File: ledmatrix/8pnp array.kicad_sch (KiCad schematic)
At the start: 8 parts

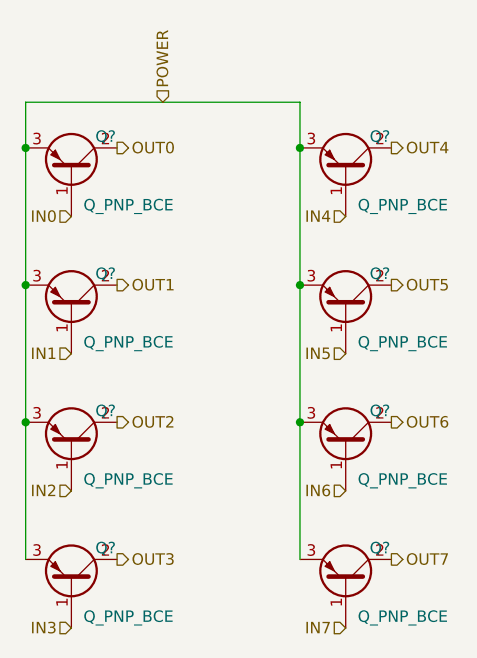
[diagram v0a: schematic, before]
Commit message: Finish ledmatrix pcb reverse engineering.
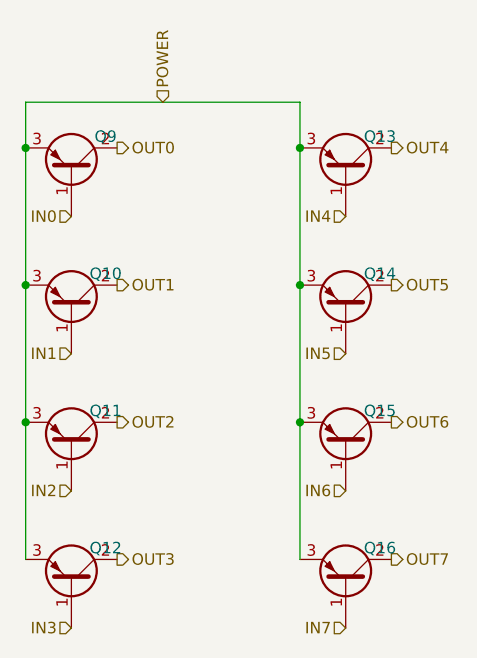
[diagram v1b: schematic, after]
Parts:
- removed Q? (x8): Q_PNP_BCE, symbol Device:Q_PNP_BCE
- added Q10, Q11, Q12, Q13, Q14, Q15, Q16, Q9: (no value), symbol Device:Q_PNP_BCE
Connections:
- net IN0: now also Q9.1 (B)
- net IN1: now also Q10.1 (B)
- net IN2: now also Q11.1 (B)
- net IN3: now also Q12.1 (B)
- net IN4: now also Q13.1 (B)
- net IN5: now also Q14.1 (B)
- net IN6: now also Q15.1 (B)
- net IN7: now also Q16.1 (B)
- net OUT0: now also Q9.2 (C)
- net OUT1: now also Q10.2 (C)
- net OUT2: now also Q11.2 (C)
- net OUT3: now also Q12.2 (C)
- net OUT4: now also Q13.2 (C)
- net OUT5: now also Q14.2 (C)
- net OUT6: now also Q15.2 (C)
- net OUT7: now also Q16.2 (C)
- net POWER: now also Q10.3 (E), Q11.3 (E), Q12.3 (E), Q13.3 (E), Q14.3 (E), Q15.3 (E), Q16.3 (E), Q9.3 (E)
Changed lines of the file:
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@@
     (effects (font (size 1.27 1.27)) (justify right))
+  )
+  (symbol (lib_id "Device:Q_PNP_BCE") (at 123.19 44.45 270) (mirror x) (unit 1)
+    (in_bom yes) (on_board yes)
+    (property "Reference" "Q13" (id 0) (at 127 40.64 90))
+    (property "Value" "" (id 1) (at 129.54 48.26 90))
+    (property "Footprint" "" (id 2) (at 125.73 39.37 0)
+      (effects (font (size 1.27 1.27)) hide)
+    )
+    (property "Datasheet" "~" (id 3) (at 123.19 44.45 0)
+      (effects (font (size 1.27 1.27)) hide)
+    )
+    (pin "1")
+    (pin "2")
+    (pin "3")
+  )
+  (symbol (lib_id "Device:Q_PNP_BCE") (at 123.19 59.69 270) (mirror x) (unit 1)
+    (in_bom yes) (on_board yes)
+    (property "Reference" "Q14" (id 0) (at 127 55.88 90))
+    (property "Value" "" (id 1) (at 129.54 63.5 90))
+    (property "Footprint" "" (id 2) (at 125.73 54.61 0)
+      (effects (font (size 1.27 1.27)) hide)
+    )
+    (property "Datasheet" "~" (id 3) (at 123.19 59.69 0)
+      (effects (font (size 1.27 1.27)) hide)
+    )
+    (pin "1")
+    (pin "2")
+    (pin "3")
+  )
+  (symbol (lib_id "Device:Q_PNP_BCE") (at 123.19 90.17 270) (mirror x) (unit 1)
+    (in_bom yes) (on_board yes)
+    (property "Reference" "Q16" (id 0) (at 127 86.36 90))
+    (property "Value" "" (id 1) (at 129.54 93.98 90))
+    (property "Footprint" "" (id 2) (at 125.73 85.09 0)
+      (effects (font (size 1.27 1.27)) hide)
+    )
+    (property "Datasheet" "~" (id 3) (at 123.19 90.17 0)
+      (effects (font (size 1.27 1.27)) hide)
+    )
+    (pin "1")
+    (pin "2")
+    (pin "3")
   )
   (symbol (lib_id "Device:Q_PNP_BCE") (at 92.71 44.45 270) (mirror x) (unit 1)
     (in_bom yes) (on_board yes)
-    (property "Reference" "Q?" (id 0) (at 96.52 40.64 90))
-    (property "Value" "Q_PNP_BCE" (id 1) (at 99.06 48.26 90))
+    (property "Reference" "Q9" (id 0) (at 96.52 40.64 90))
+    (property "Value" "" (id 1) (at 99.06 48.26 90))
     (property "Footprint" "" (id 2) (at 95.25 39.37 0)
       (effects (font (size 1.27 1.27)) hide)
@@
     (pin "3")
   )
-  (symbol (lib_id "Device:Q_PNP_BCE") (at 123.19 59.69 270) (mirror x) (unit 1)
+  (symbol (lib_id "Device:Q_PNP_BCE") (at 92.71 90.17 270) (mirror x) (unit 1)
     (in_bom yes) (on_board yes)
-    (property "Reference" "Q?" (id 0) (at 127 55.88 90))
-    (property "Value" "Q_PNP_BCE" (id 1) (at 129.54 63.5 90))
-    (property "Footprint" "" (id 2) (at 125.73 54.61 0)
+    (property "Reference" "Q12" (id 0) (at 96.52 86.36 90))
+    (property "Value" "" (id 1) (at 99.06 93.98 90))
+    (property "Footprint" "" (id 2) (at 95.25 85.09 0)
       (effects (font (size 1.27 1.27)) hide)
     )
-    (property "Datasheet" "~" (id 3) (at 123.19 59.69 0)
-      (effects (font (size 1.27 1.27)) hide)
-    )
-    (pin "1")
-    (pin "2")
-    (pin "3")
-  )
-  (symbol (lib_id "Device:Q_PNP_BCE") (at 92.71 74.93 270) (mirror x) (unit 1)
-    (in_bom yes) (on_board yes)
-    (property "Reference" "Q?" (id 0) (at 96.52 71.12 90))
-    (property "Value" "Q_PNP_BCE" (id 1) (at 99.06 78.74 90))
-    (property "Footprint" "" (id 2) (at 95.25 69.85 0)
-      (effects (font (size 1.27 1.27)) hide)
-    )
-    (property "Datasheet" "~" (id 3) (at 92.71 74.93 0)
+    (property "Datasheet" "~" (id 3) (at 92.71 90.17 0)
       (effects (font (size 1.27 1.27)) hide)
     )
@@
   (symbol (lib_id "Device:Q_PNP_BCE") (at 92.71 59.69 270) (mirror x) (unit 1)
     (in_bom yes) (on_board yes)
-    (property "Reference" "Q?" (id 0) (at 96.52 55.88 90))
-    (property "Value" "Q_PNP_BCE" (id 1) (at 99.06 63.5 90))
+    (property "Reference" "Q10" (id 0) (at 96.52 55.88 90))
+    (property "Value" "" (id 1) (at 99.06 63.5 90))
     (property "Footprint" "" (id 2) (at 95.25 54.61 0)
       (effects (font (size 1.27 1.27)) hide)
@@
     (pin "3")
   )
-  (symbol (lib_id "Device:Q_PNP_BCE") (at 92.71 90.17 270) (mirror x) (unit 1)
-    (in_bom yes) (on_board yes)
-    (property "Reference" "Q?" (id 0) (at 96.52 86.36 90))
-    (property "Value" "Q_PNP_BCE" (id 1) (at 99.06 93.98 90))
-    (property "Footprint" "" (id 2) (at 95.25 85.09 0)
-      (effects (font (size 1.27 1.27)) hide)
-    )
-    (property "Datasheet" "~" (id 3) (at 92.71 90.17 0)
-      (effects (font (size 1.27 1.27)) hide)
-    )
-    (pin "1")
-    (pin "2")
-    (pin "3")
-  )
-  (symbol (lib_id "Device:Q_PNP_BCE") (at 123.19 90.17 270) (mirror x) (unit 1)
-    (in_bom yes) (on_board yes)
-    (property "Reference" "Q?" (id 0) (at 127 86.36 90))
-    (property "Value" "Q_PNP_BCE" (id 1) (at 129.54 93.98 90))
-    (property "Footprint" "" (id 2) (at 125.73 85.09 0)
-      (effects (font (size 1.27 1.27)) hide)
-    )
-    (property "Datasheet" "~" (id 3) (at 123.19 90.17 0)
-      (effects (font (size 1.27 1.27)) hide)
-    )
-    (pin "1")
-    (pin "2")
-    (pin "3")
-  )
   (symbol (lib_id "Device:Q_PNP_BCE") (at 123.19 74.93 270) (mirror x) (unit 1)
     (in_bom yes) (on_board yes)
-    (property "Reference" "Q?" (id 0) (at 127 71.12 90))
-    (property "Value" "Q_PNP_BCE" (id 1) (at 129.54 78.74 90))
+    (property "Reference" "Q15" (id 0) (at 127 71.12 90))
+    (property "Value" "" (id 1) (at 129.54 78.74 90))
     (property "Footprint" "" (id 2) (at 125.73 69.85 0)
       (effects (font (size 1.27 1.27)) hide)
@@
     (pin "3")
   )
-  (symbol (lib_id "Device:Q_PNP_BCE") (at 123.19 44.45 270) (mirror x) (unit 1)
+  (symbol (lib_id "Device:Q_PNP_BCE") (at 92.71 74.93 270) (mirror x) (unit 1)
     (in_bom yes) (on_board yes)
-    (property "Reference" "Q?" (id 0) (at 127 40.64 90))
-    (property "Value" "Q_PNP_BCE" (id 1) (at 129.54 48.26 90))
-    (property "Footprint" "" (id 2) (at 125.73 39.37 0)
+    (property "Reference" "Q11" (id 0) (at 96.52 71.12 90))
+    (property "Value" "" (id 1) (at 99.06 78.74 90))
+    (property "Footprint" "" (id 2) (at 95.25 69.85 0)
       (effects (font (size 1.27 1.27)) hide)
     )
-    (property "Datasheet" "~" (id 3) (at 123.19 44.45 0)
+    (property "Datasheet" "~" (id 3) (at 92.71 74.93 0)
       (effects (font (size 1.27 1.27)) hide)
     )

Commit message: switch to desktop
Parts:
- Q10, Q11, Q12, Q13, Q14, Q15, Q16, Q9: value (none) -> ~
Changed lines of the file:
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@@
     (in_bom yes) (on_board yes)
     (property "Reference" "Q13" (id 0) (at 127 40.64 90))
-    (property "Value" "" (id 1) (at 129.54 48.26 90))
+    (property "Value" "~" (id 1) (at 129.54 48.26 90))
     (property "Footprint" "" (id 2) (at 125.73 39.37 0)
       (effects (font (size 1.27 1.27)) hide)
@@
     (in_bom yes) (on_board yes)
     (property "Reference" "Q14" (id 0) (at 127 55.88 90))
-    (property "Value" "" (id 1) (at 129.54 63.5 90))
+    (property "Value" "~" (id 1) (at 129.54 63.5 90))
     (property "Footprint" "" (id 2) (at 125.73 54.61 0)
       (effects (font (size 1.27 1.27)) hide)
@@
     (in_bom yes) (on_board yes)
     (property "Reference" "Q16" (id 0) (at 127 86.36 90))
-    (property "Value" "" (id 1) (at 129.54 93.98 90))
+    (property "Value" "~" (id 1) (at 129.54 93.98 90))
     (property "Footprint" "" (id 2) (at 125.73 85.09 0)
       (effects (font (size 1.27 1.27)) hide)
@@
     (in_bom yes) (on_board yes)
     (property "Reference" "Q9" (id 0) (at 96.52 40.64 90))
-    (property "Value" "" (id 1) (at 99.06 48.26 90))
+    (property "Value" "~" (id 1) (at 99.06 48.26 90))
     (property "Footprint" "" (id 2) (at 95.25 39.37 0)
       (effects (font (size 1.27 1.27)) hide)
@@
     (in_bom yes) (on_board yes)
     (property "Reference" "Q12" (id 0) (at 96.52 86.36 90))
-    (property "Value" "" (id 1) (at 99.06 93.98 90))
+    (property "Value" "~" (id 1) (at 99.06 93.98 90))
     (property "Footprint" "" (id 2) (at 95.25 85.09 0)
       (effects (font (size 1.27 1.27)) hide)
@@
     (in_bom yes) (on_board yes)
     (property "Reference" "Q10" (id 0) (at 96.52 55.88 90))
-    (property "Value" "" (id 1) (at 99.06 63.5 90))
+    (property "Value" "~" (id 1) (at 99.06 63.5 90))
     (property "Footprint" "" (id 2) (at 95.25 54.61 0)
       (effects (font (size 1.27 1.27)) hide)
@@
     (in_bom yes) (on_board yes)
     (property "Reference" "Q15" (id 0) (at 127 71.12 90))
-    (property "Value" "" (id 1) (at 129.54 78.74 90))
+    (property "Value" "~" (id 1) (at 129.54 78.74 90))
     (property "Footprint" "" (id 2) (at 125.73 69.85 0)
       (effects (font (size 1.27 1.27)) hide)
@@
     (in_bom yes) (on_board yes)
     (property "Reference" "Q11" (id 0) (at 96.52 71.12 90))
-    (property "Value" "" (id 1) (at 99.06 78.74 90))
+    (property "Value" "~" (id 1) (at 99.06 78.74 90))
     (property "Footprint" "" (id 2) (at 95.25 69.85 0)
       (effects (font (size 1.27 1.27)) hide)
